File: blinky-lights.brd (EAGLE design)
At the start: 63.5 x 63.5 mm, 20 parts, among them Q1 N3, U1 555, U2 A2678EAT

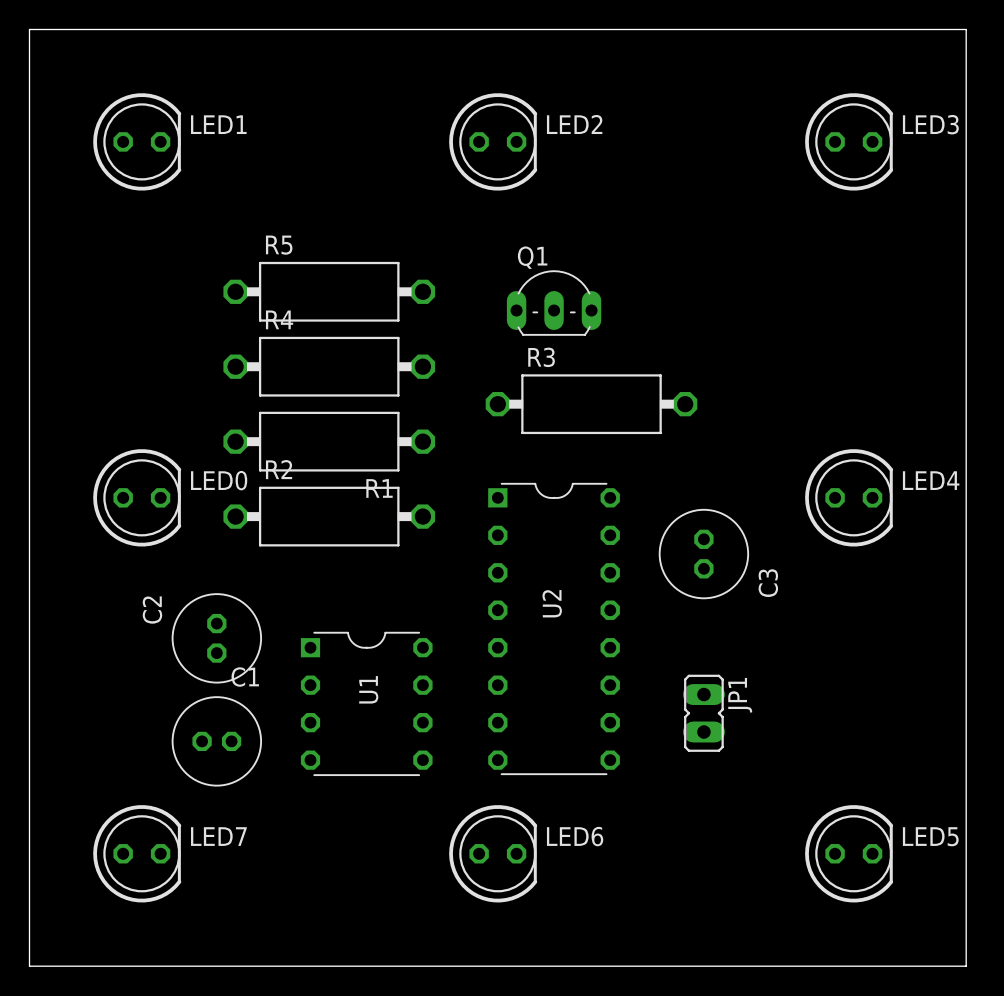
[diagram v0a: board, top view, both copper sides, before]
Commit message: board layout
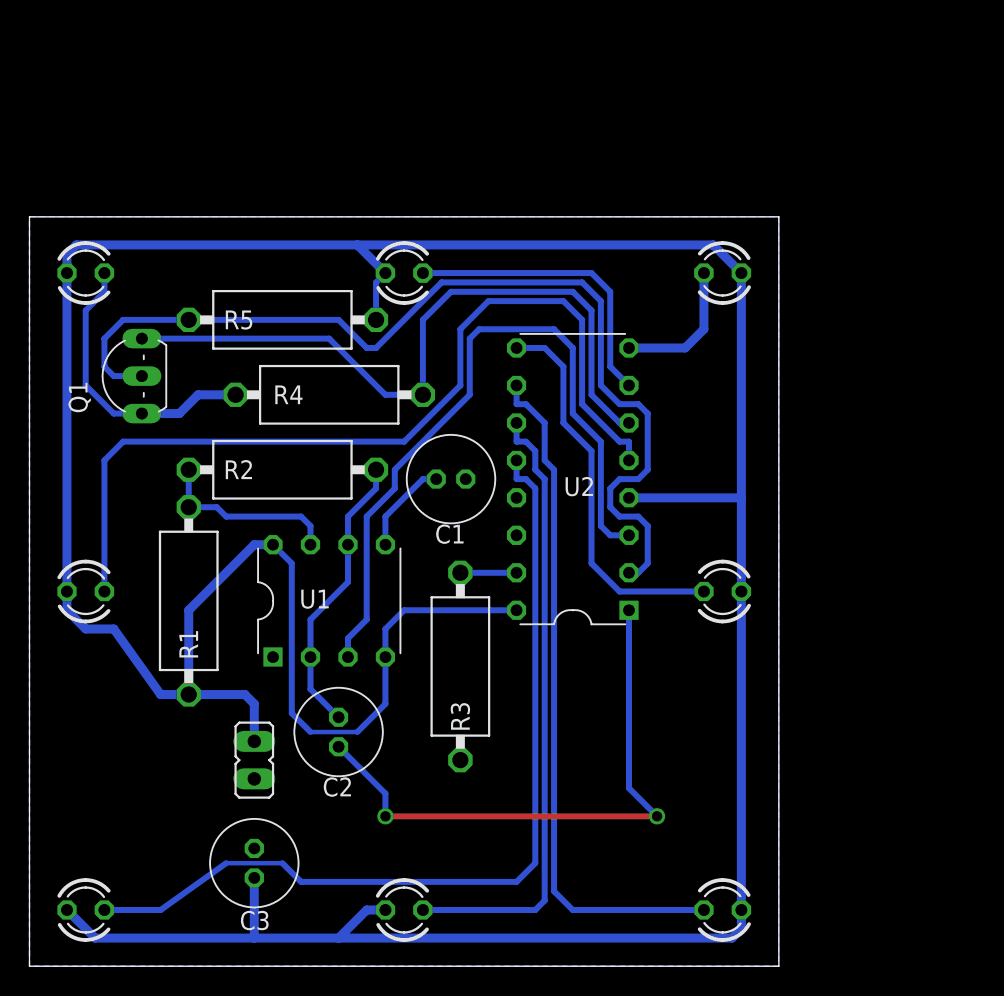
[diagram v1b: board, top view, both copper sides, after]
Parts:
- C1: value 10n -> 0.01u
- C3: value 100u -> 10u
- LED0, LED1, LED2, LED3, LED4, LED5, LED6, LED7: device led:LED5MM -> led:LED3MM
- Q1: value N3 -> NFET
- R4: value 1k -> 50
- R5: value 10k -> 1k
- moved C3 37.0 mm to (15.2, 6.99)
- moved JP1 30.6 mm to (15.2, 14.0), turned to 0 degrees
- moved Q1 29.8 mm to (6.35, 40.0), turned to 90 degrees
- moved C1 23.8 mm to (28.6, 33.0), turned to 0 degrees
- moved R3 19.9 mm to (29.2, 20.3), turned to 90 degrees
- moved R1 14.4 mm to (10.8, 24.8), turned to 270 degrees
- moved LED3 12.6 mm to (47.0, 47.0), turned to 180 degrees
- moved LED2 10.9 mm to (25.4, 47.0)
- moved LED4 10.9 mm to (47.0, 25.4), turned to 180 degrees
- moved C2 10.4 mm to (21.0, 15.9)
- moved U2 10.2 mm to (36.8, 33.0), turned to 90 degrees
- moved LED1 9.67 mm to (3.81, 47.0)
- moved LED5 9.67 mm to (47.0, 3.81), turned to 180 degrees
- moved U1 7.43 mm to (20.3, 24.8), turned to 0 degrees
- moved LED0 7.41 mm to (3.81, 25.4)
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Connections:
- removed net DATA: Q1.E, R4.2, U2.2
- removed net N$12: Q1.B, R5.2
- removed net N$13: C3.A, JP1.1
- new net N$5: Q1.S, R4.2, U2.6
- new net SENSE: LED1.K, Q1.G, R4.1
- net FEEDBACK: now also Q1.D, R5.2, U2.2; no longer LED1.K, R5.1, U2.6
- net GND: now also JP1.1; no longer R4.1
- net VCC: now also C3.A, R5.1; no longer Q1.C
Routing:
- net VCC: track 0.00 -> 249.6 mm
- net FEEDBACK: track 0.00 -> 67.0 mm
- net N$1: track 0.00 -> 59.7 mm
- net N$4: track 0.00 -> 59.5 mm
- net CLK: track 0.00 -> 47.8 mm
- net N$5: track 0.00 -> 47.5 mm
- net N$7: track 0.00 -> 46.4 mm
- net N$8: track 0.00 -> 42.1 mm
- net GND: track 0.00 -> 39.2 mm, vias 0 -> 2
- net N$3: track 0.00 -> 26.2 mm
- net N$2: track 0.00 -> 20.1 mm
- net SENSE: track 0.00 -> 19.6 mm
- net N$11: track 0.00 -> 19.4 mm
- net N$9: track 0.00 -> 12.6 mm
- net N$6: track 0.00 -> 9.42 mm
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- added copper zone on layer 16, net GND
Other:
- board size 63.5 x 63.5 mm -> 50.8 x 50.8 mm
